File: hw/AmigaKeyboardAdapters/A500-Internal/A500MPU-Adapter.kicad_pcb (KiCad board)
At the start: 2 copper layers, 24.1 x 30.5 mm, 15 parts, among them P1 CONN_01X08, P2 CONN_01X08, P3 CONN_02X03, P4 CONN_01X02, P5 CONN_01X02

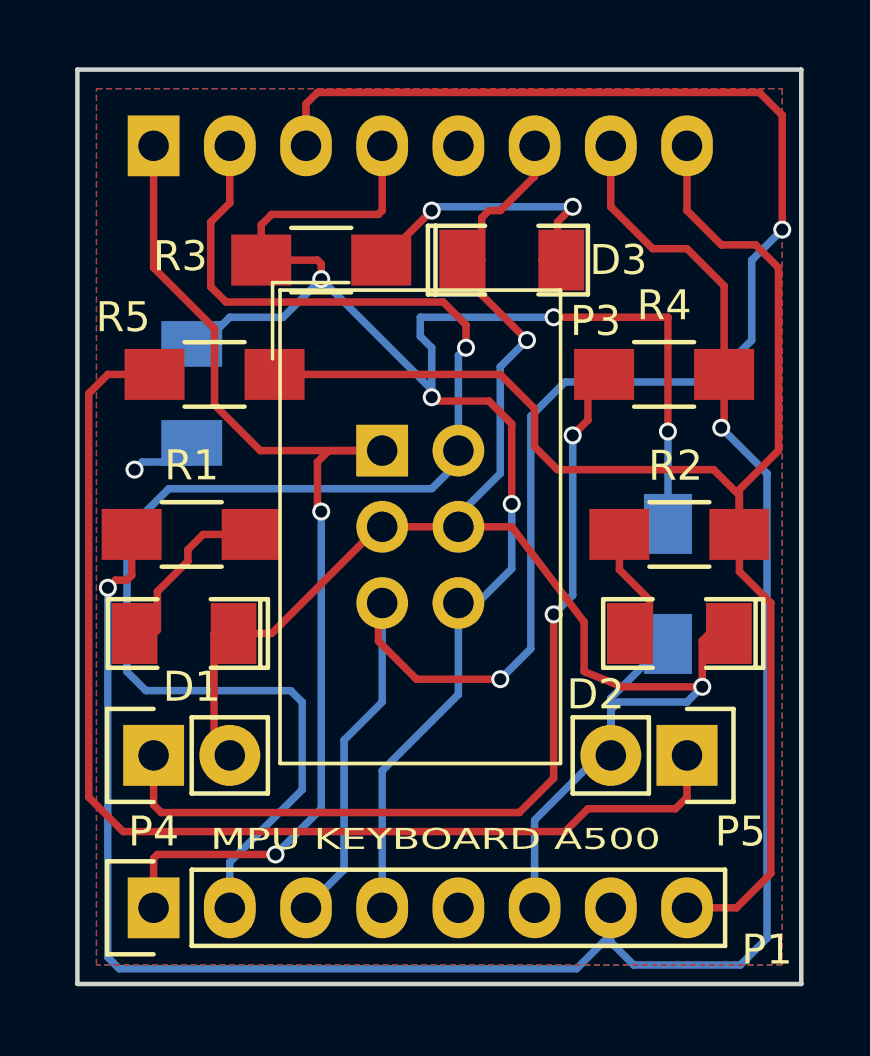
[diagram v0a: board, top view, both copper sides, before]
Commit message: From KiCAD 4 to KiCAD 5
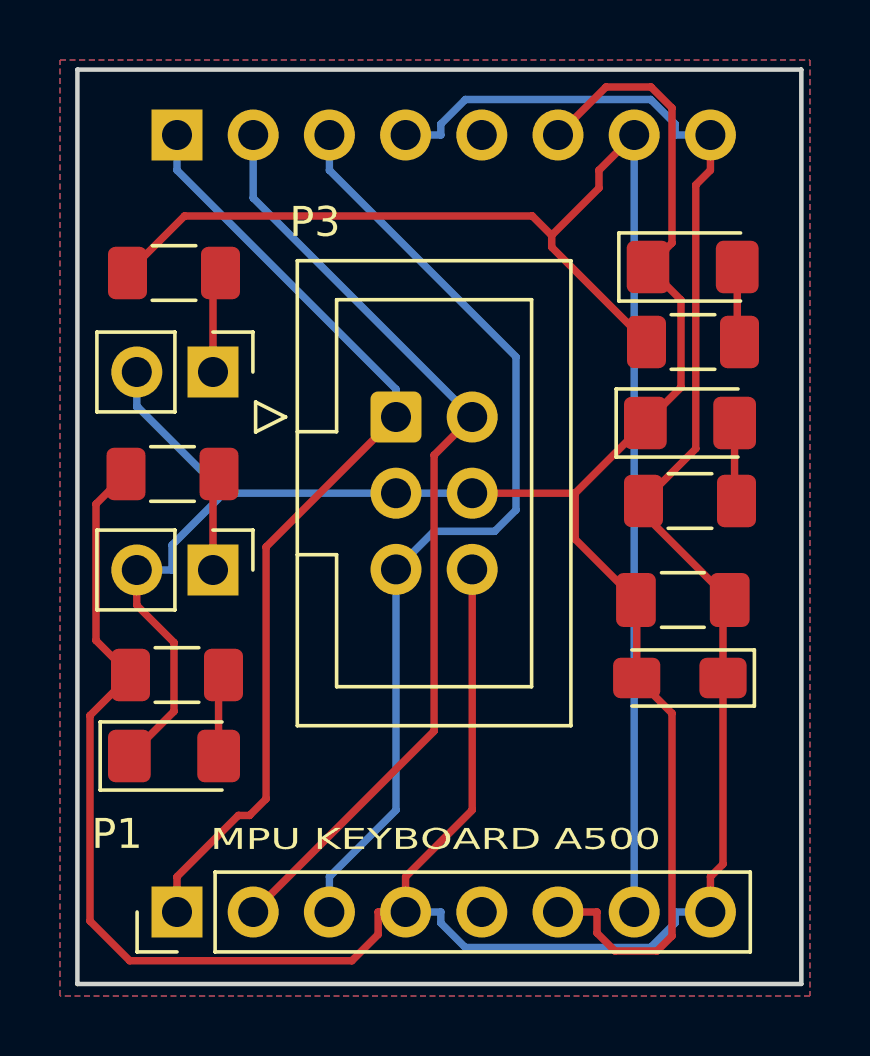
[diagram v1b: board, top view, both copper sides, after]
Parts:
- C1: footprint SMD_Packages:SMD-1206_Pol -> Capacitor_Tantalum_SMD:CP_EIA-3216-12_Kemet-S_Pad1.58x1.35mm_HandSolder; moved to F.Cu
- C2: footprint Capacitors_SMD:C_1206_HandSoldering -> Capacitor_SMD:C_1206_3216Metric_Pad1.33x1.80mm_HandSolder; moved to F.Cu
- D1: value LED GREEN -> POWER ORANGE; footprint SMD_Packages:SMD-1206_Pol -> LED_SMD:LED_1206_3216Metric_Pad1.42x1.75mm_HandSolder
- D2: value DISK YELLOW -> FLOPPY GREEN; footprint SMD_Packages:SMD-1206_Pol -> LED_SMD:LED_1206_3216Metric_Pad1.42x1.75mm_HandSolder
- D3: footprint SMD_Packages:SMD-1206_Pol -> LED_SMD:LED_1206_3216Metric_Pad1.42x1.75mm_HandSolder
- P1: value CONN_01X08 -> Conn_01x08; footprint Pin_Headers:Pin_Header_Straight_1x08 -> Connector_PinHeader_2.54mm:PinHeader_1x08_P2.54mm_Vertical
- P2: value CONN_01X08 -> Conn_01x08; footprint Socket_Strips:Socket_Strip_Straight_1x08 -> Connector_PinSocket_2.54mm:PinSocket_1x08_P2.54mm_Vertical
- P3: value CONN_02X03 -> Conn_02x03; footprint RetroBitLab:IDC-Header_2x03_P2.54mm_Vertical -> Connector_IDC:IDC-Header_2x03_P2.54mm_Vertical
- P4, P5: value CONN_01X02 -> Conn_01x02; footprint Pin_Headers:Pin_Header_Straight_1x02 -> Connector_PinHeader_2.54mm:PinHeader_1x02_P2.54mm_Vertical
- R1, R2, R3, R4, R5: value 330 -> 330R; footprint Resistors_SMD:R_1206_HandSoldering -> Resistor_SMD:R_1206_3216Metric_Pad1.30x1.75mm_HandSolder
- moved D1 20.9 mm to (165.3, 103.1), turned to 0 degrees
- moved D3 20.0 mm to (148.0, 119.4)
- moved C1 18.8 mm to (164.9, 116.8), turned to 180 degrees
- moved R1 17.9 mm to (165.3, 105.6)
- moved P5 17.0 mm to (149.3, 113.2)
- moved R4 16.7 mm to (148.0, 103.3)
- moved R3 14.6 mm to (148.1, 116.7)
- moved P4 12.9 mm to (149.3, 106.6), turned to 270 degrees
- moved D2 7.02 mm to (165.2, 108.3), turned to 0 degrees
- moved R5 3.60 mm to (147.9, 110.0)
- moved P3 1.21 mm to (155.4, 108.1)
- moved R2 1.17 mm to (165.2, 110.9), turned to 0 degrees
- moved P2 0.86 mm to (148.1, 98.7), turned to 270 degrees
- moved P1 0.79 mm to (148.1, 124.6)
- moved C2 0.73 mm to (165.0, 114.2), turned to 180 degrees
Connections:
- C1 pad 1: VCC -> INUSE
- C2 pad 1: VCC -> INUSE
- P1 pad 4: VCC -> INUSE
- P1 pad 5: (no net) -> Net-(P1-Pad5)
- P2 pad 4: VCC -> INUSE
- P2 pad 5: (no net) -> Net-(P2-Pad5)
- P3 pad 6: VCC -> INUSE
- R3 pad 1: VCC -> INUSE
- R4 pad 1: Net-(P4-Pad1) -> STATUS
- R4 pad 2: STATUS -> Net-(P4-Pad1)
- R5 pad 1: Net-(P5-Pad1) -> INUSE
- R5 pad 2: INUSE -> Net-(P5-Pad1)
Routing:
- net VCC: track 60.5 -> 0.00 mm, vias 5 -> 0
- net INUSE: track 49.6 -> 92.3 mm
- net Net-(P5-Pad1): track 38.2 -> 3.28 mm
- net RESET: track 60.4 -> 32.2 mm, vias 2 -> 0
- net Net-(P4-Pad1): track 29.7 -> 3.40 mm, vias 2 -> 0
- net STATUS: track 69.3 -> 50.4 mm, vias 2 -> 0
- net DATA: track 49.5 -> 31.9 mm, vias 1 -> 0
- net GND: track 60.3 -> 69.6 mm, vias 3 -> 0
- net Net-(D3-Pad2): track 9.32 -> 2.77 mm, vias 2 -> 0
- net CLOCK: track 37.5 -> 32.2 mm, vias 2 -> 0
- net Net-(D1-Pad2): track 5.60 -> 2.53 mm
- net Net-(D2-Pad2): track 3.72 -> 2.63 mm
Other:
- rule pad_to_mask_clearance: 0.2 -> 0
- board text added: "designed by R.G.2018/2022"
- board text removed: "designed by R.G.2018"
